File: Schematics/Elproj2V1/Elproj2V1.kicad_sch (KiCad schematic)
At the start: 22 parts, among them J1 Conn_01x04_Pin, J2 Conn_01x04_Pin, J3 Conn_01x04_Pin, J4 Conn_01x04_Pin, J5 Conn_01x04_Pin, Q1 PMOS, Q2 NMOS, SW2 Manual, U1 MOUDLE-SEEEDUINO-XIAO-ESP32C3

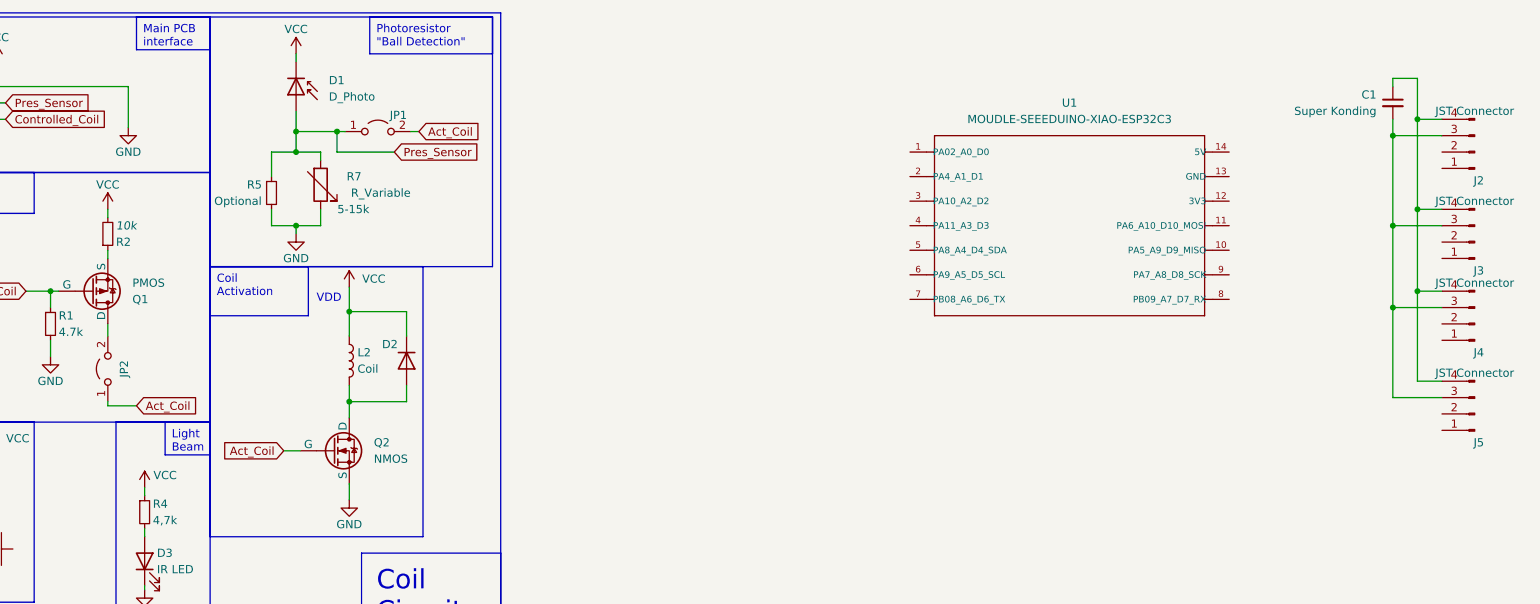
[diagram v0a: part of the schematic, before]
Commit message: Update Elproj2V1.kicad_sch
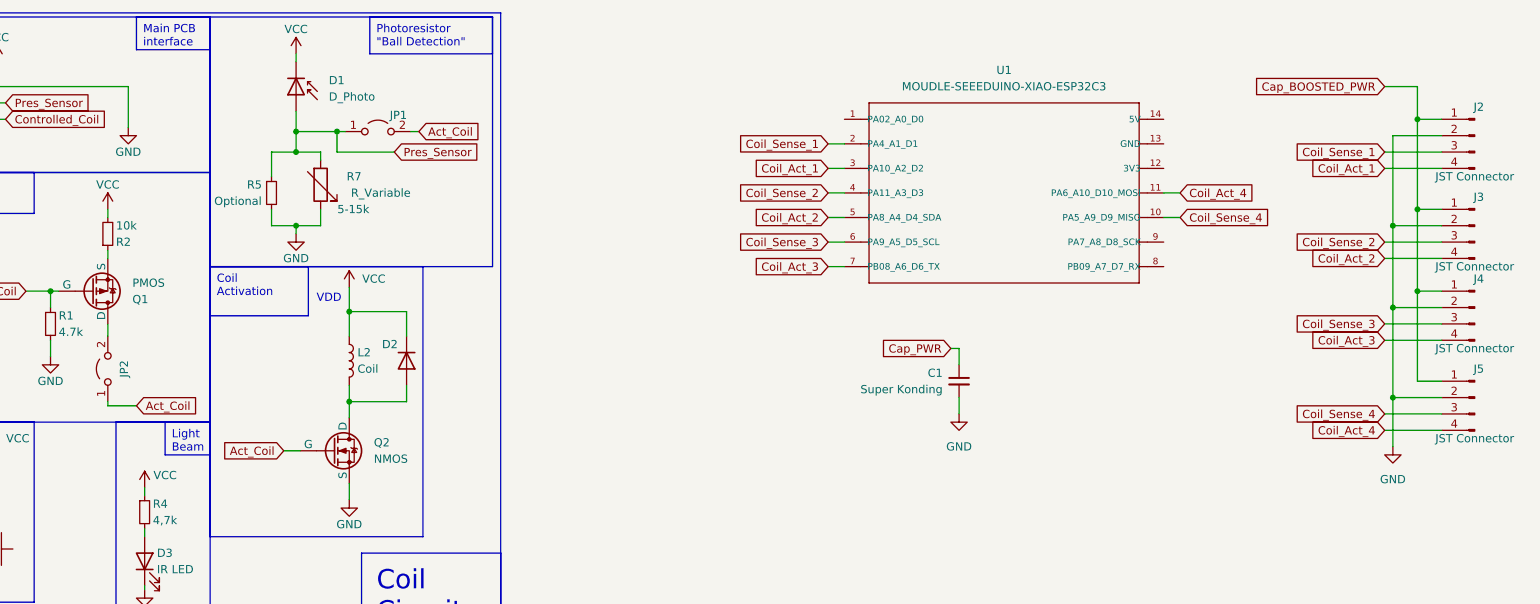
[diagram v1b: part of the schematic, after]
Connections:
- net GND: now also C1.2, J2.2 (Pin_2), J3.2 (Pin_2), J4.2 (Pin_2), J5.2 (Pin_2)
- net Cap_BOOSTED_PWR: now reaches J3.1 (Pin_1)
- net Cap_BOOSTED_PWR: now also J2.1 (Pin_1), J4.1 (Pin_1), J5.1 (Pin_1)
- net Coil_Sense_4: now reaches U1.10 (PA5_A9_D9_MISO)
- net Coil_Sense_4: now also J5.3 (Pin_3)
- net Coil_Act_4: now reaches U1.11 (PA6_A10_D10_MOSI)
- net Coil_Act_4: now also J5.4 (Pin_4)
- net Coil_Sense_1: now reaches U1.2 (PA4_A1_D1)
- net Coil_Sense_1: now also J2.3 (Pin_3)
- net Coil_Act_1: now reaches U1.3 (PA10_A2_D2)
- net Coil_Act_1: now also J2.4 (Pin_4)
- net Coil_Sense_2: now reaches U1.4 (PA11_A3_D3)
- net Coil_Sense_2: now also J3.3 (Pin_3)
- net Coil_Act_2: now reaches U1.5 (PA8_A4_D4_SDA)
- net Coil_Act_2: now also J3.4 (Pin_4)
- net Coil_Sense_3: now reaches U1.6 (PA9_A5_D5_SCL)
- net Coil_Sense_3: now also J4.3 (Pin_3)
- net Coil_Act_3: now reaches U1.7 (PB08_A6_D6_TX)
- net Coil_Act_3: now also J4.4 (Pin_4)
- new net Cap_PWR: C1.1
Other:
- moved on the sheet: J2, U1

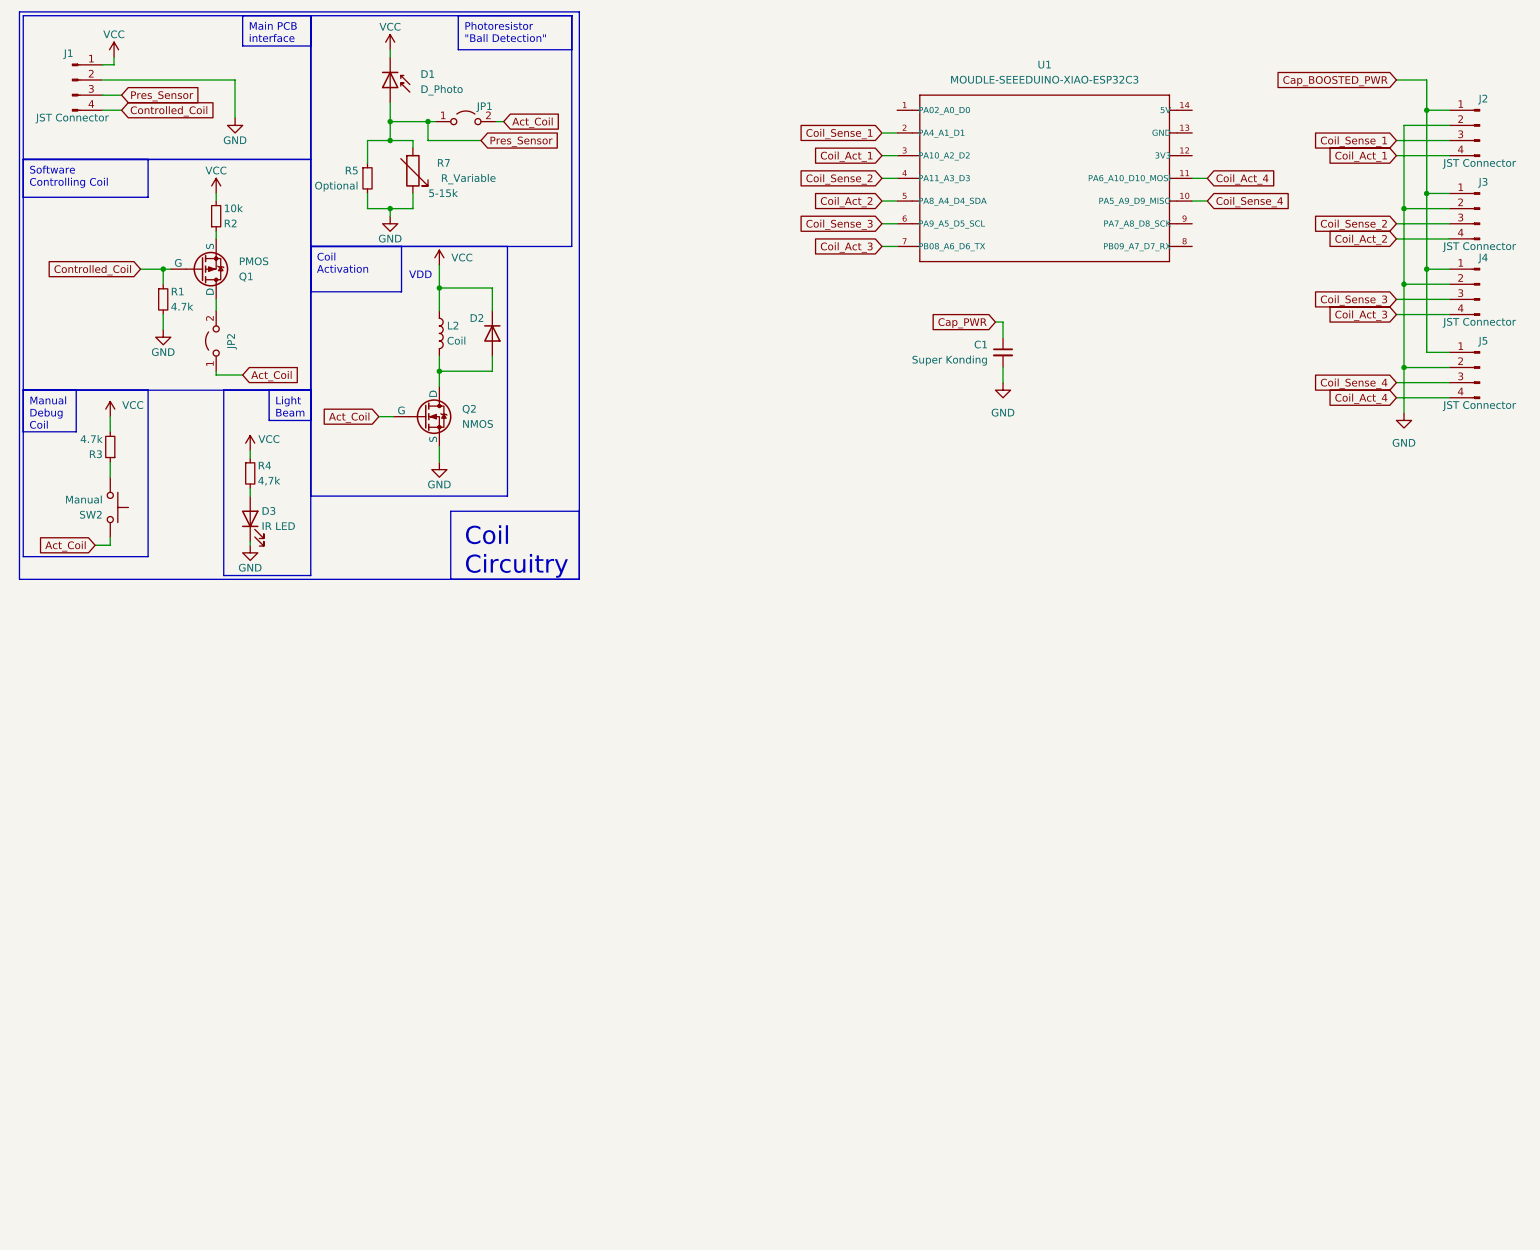
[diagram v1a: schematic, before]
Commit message: starting buck stuff
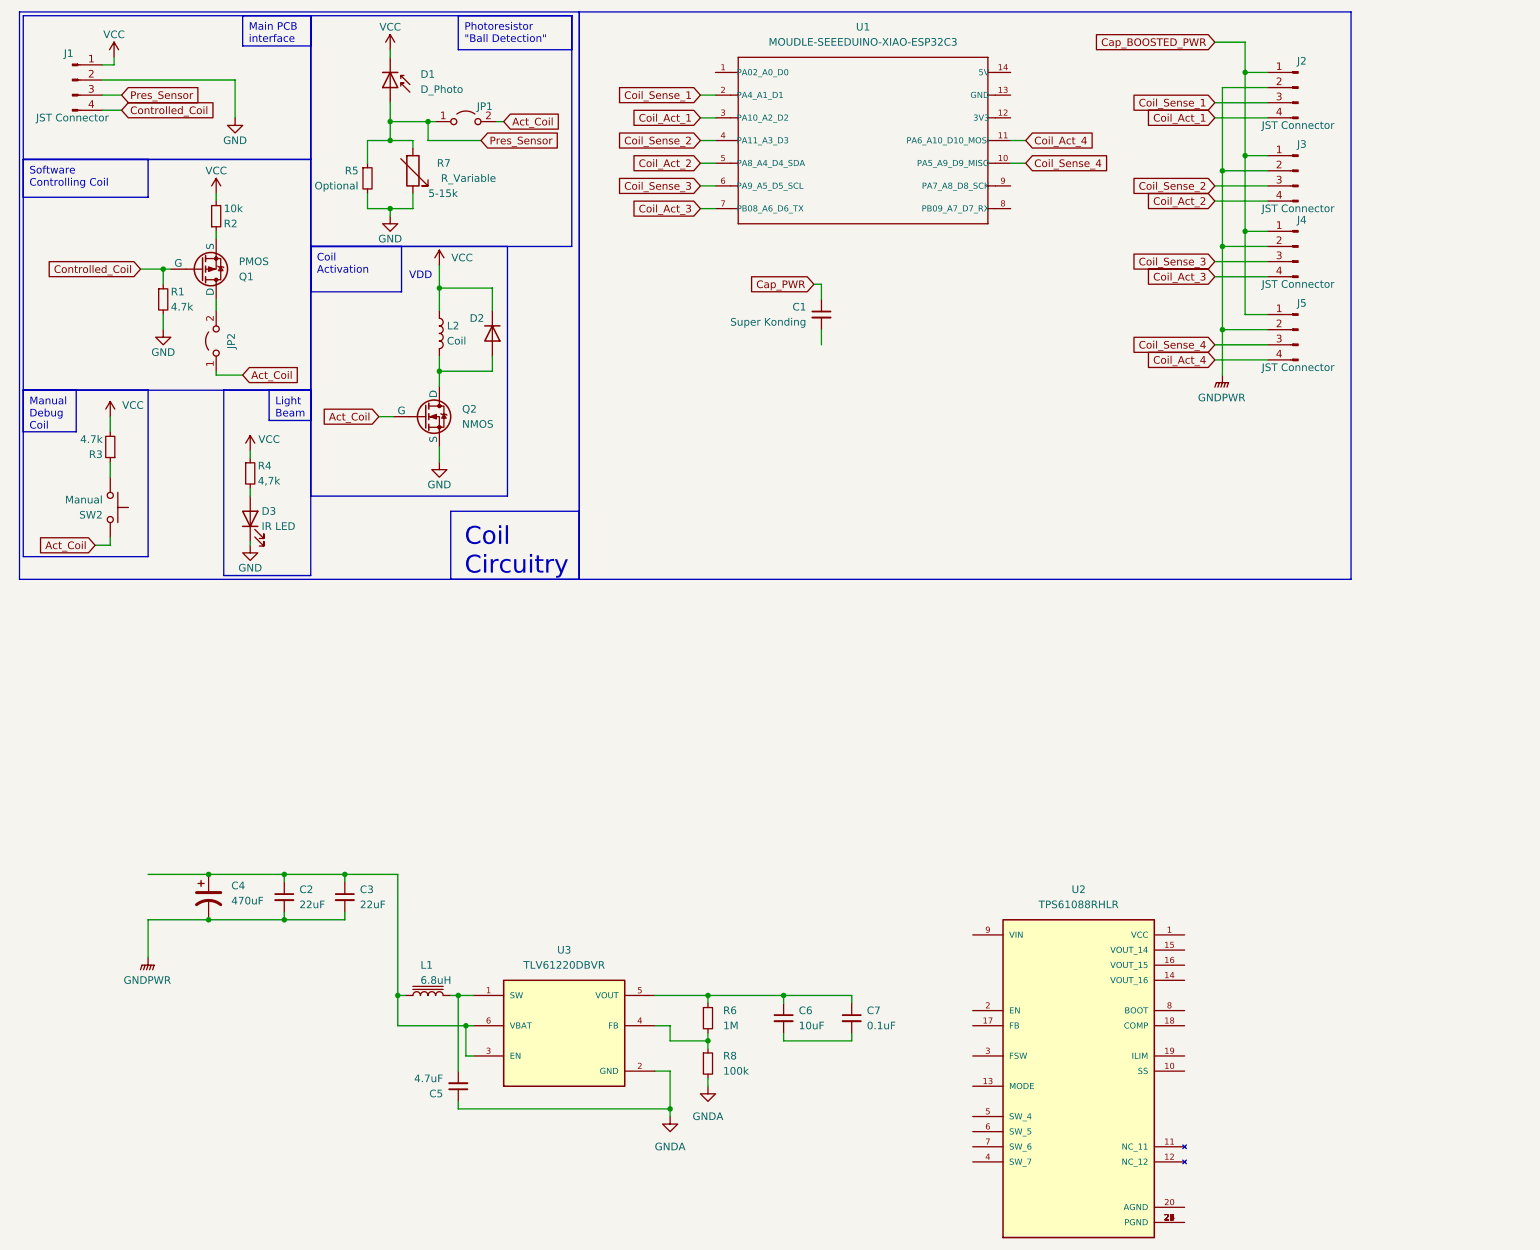
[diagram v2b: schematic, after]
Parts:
- added C2, C3: 22uF, symbol Device:C_Small
- added C4: 470uF, symbol Device:C_Polarized_US
- added C5: 4.7uF, symbol Device:C_Small
- added C6: 10uF, symbol Device:C_Small
- added C7: 0.1uF, symbol Device:C_Small
- added L1: 6.8uH, symbol Device:L_Iron
- added R6: 1M, symbol Device:R_Small
- added R8: 100k, symbol Device:R_Small
- added U2: TPS61088RHLR, TPS61088RHLR:IC_TPS61088RHLR, symbol TPS61088RHLR:TPS61088RHLR
- added U3: TLV61220DBVR, TLV61220DBVR:SOT95P280X145-6N, symbol TLV61220DBVR:TLV61220DBVR
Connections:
- net GND: no longer C1.2, J2.2 (Pin_2), J3.2 (Pin_2), J4.2 (Pin_2), J5.2 (Pin_2)
- new net: C5.2, L1.1, U3.1 (SW)
- new net: C2.1, C3.1, C4.1, L1.2, U3.3 (EN), U3.6 (VBAT)
- new net: U2.21 (PGND), U2.22 (PGND), U2.23 (PGND), U2.24 (PGND), U2.25 (PGND), U2.26 (PGND), U2.27 (PGND), U2.28 (PGND), U2.29 (PGND)
- new net: C6.1, C7.1, R6.1, U3.5 (VOUT)
- new net: C6.2, C7.2
- new net: R6.2, R8.1, U3.4 (FB)
- new net GNDA: C5.1, R8.2, U3.2 (GND)
- new net GNDPWR: C2.2, C3.2, C4.2, J2.2 (Pin_2), J3.2 (Pin_2), J4.2 (Pin_2), J5.2 (Pin_2)
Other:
- moved on the sheet: C1, J2, J3, J4, J5, U1
